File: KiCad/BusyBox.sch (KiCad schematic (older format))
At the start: 6 parts, among them SW1 SW_DIP_4, U1 ESP-12F

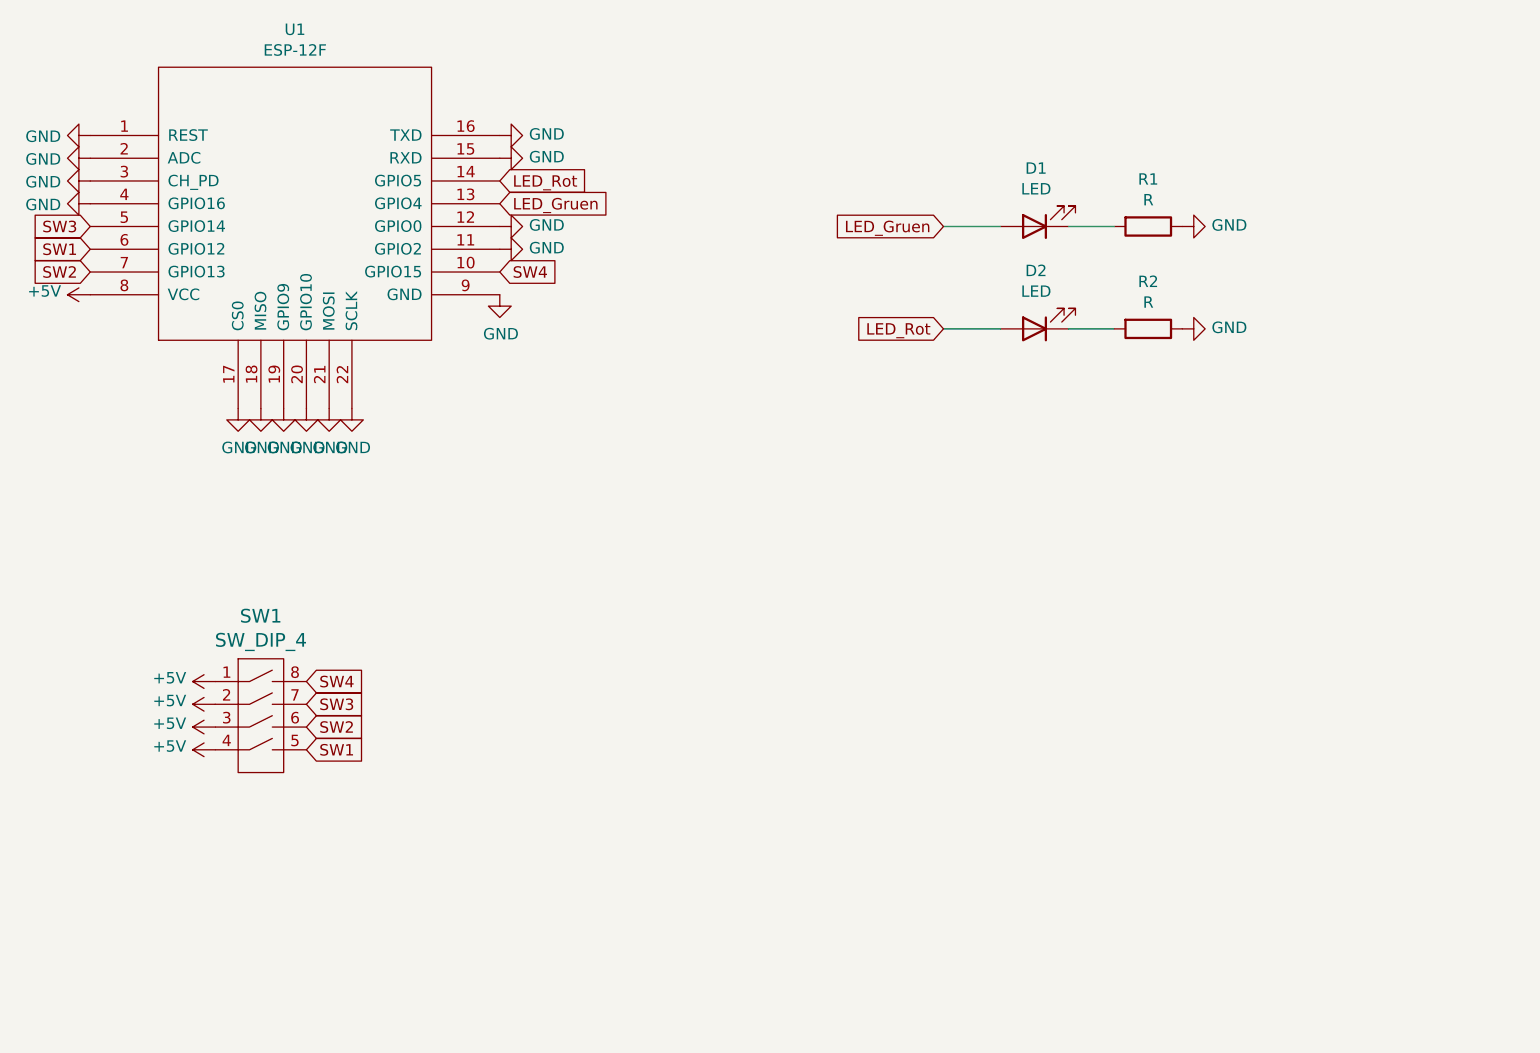
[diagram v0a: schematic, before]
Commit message: Schaltplan und Platine designed
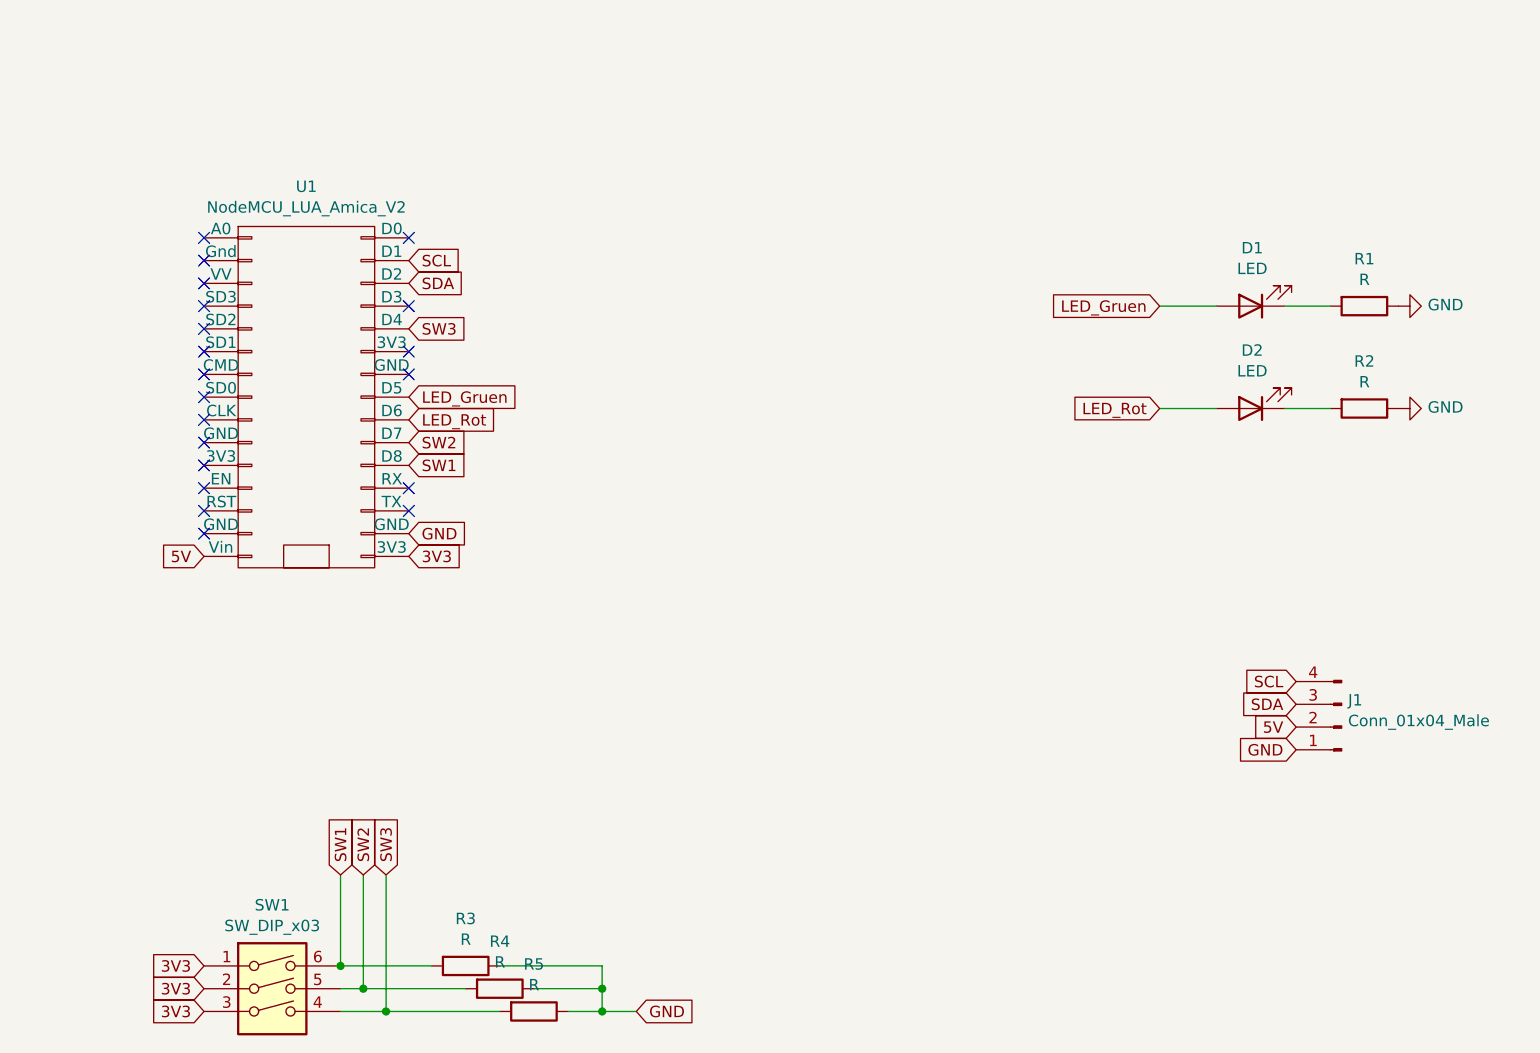
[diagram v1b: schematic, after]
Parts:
- removed SW1: SW_DIP_4, symbol kicad-library:SW_DIP_4
- removed U1: ESP-12F, symbol ESP8266:ESP-12F
- added J1: Conn_01x04_Male, Connector_PinHeader_2.54mm:PinHeader_1x04_P2.54mm_Vertical, symbol Connector:Conn_01x04_Male
- added R3, R4, R5: R, Resistor_THT:R_Axial_DIN0207_L6.3mm_D2.5mm_P10.16mm_Horizontal, symbol Device:R
- added SW1: SW_DIP_x03, Button_Switch_THT:SW_DIP_SPSTx03_Slide_9.78x9.8mm_W7.62mm_P2.54mm, symbol Switch:SW_DIP_x03
- added U1: NodeMCU_LUA_Amica_V2, ESP8266:NodeMCU-LoLinV3, symbol nodemcu:NodeMCU_LUA_Amica_V2
- D1, D2: footprint (none) -> LED_THT:LED_D5.0mm
- R1, R2: footprint (none) -> Resistor_THT:R_Axial_DIN0207_L6.3mm_D2.5mm_P10.16mm_Horizontal
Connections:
- net GND: now also J1.1 (Pin_1), R3.1, R4.1, R5.1, U1.17 (GND)
- net LED_Gruen: now also U1.23 (D5)
- net LED_Rot: now also U1.22 (D6)
- net SW1: now also R3.2, SW1.6, U1.20 (D8)
- net SW2: now also R4.2, SW1.5, U1.21 (D7)
- net SW3: now also R5.2, SW1.4, U1.26 (D4)
- new net 3V3: SW1.1, SW1.2, SW1.3, U1.16 (3V3)
- new net 5V: J1.2 (Pin_2), U1.15 (Vin)
- new net SCL: J1.4 (Pin_4), U1.29 (D1)
- new net SDA: J1.3 (Pin_3), U1.28 (D2)
- no-connect marks 0 -> 20
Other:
- moved on the sheet: D1, D2, R1, R2
